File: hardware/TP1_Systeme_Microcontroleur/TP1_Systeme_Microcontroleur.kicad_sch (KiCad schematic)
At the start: 11 parts, among them U1 STM32L021K4Tx

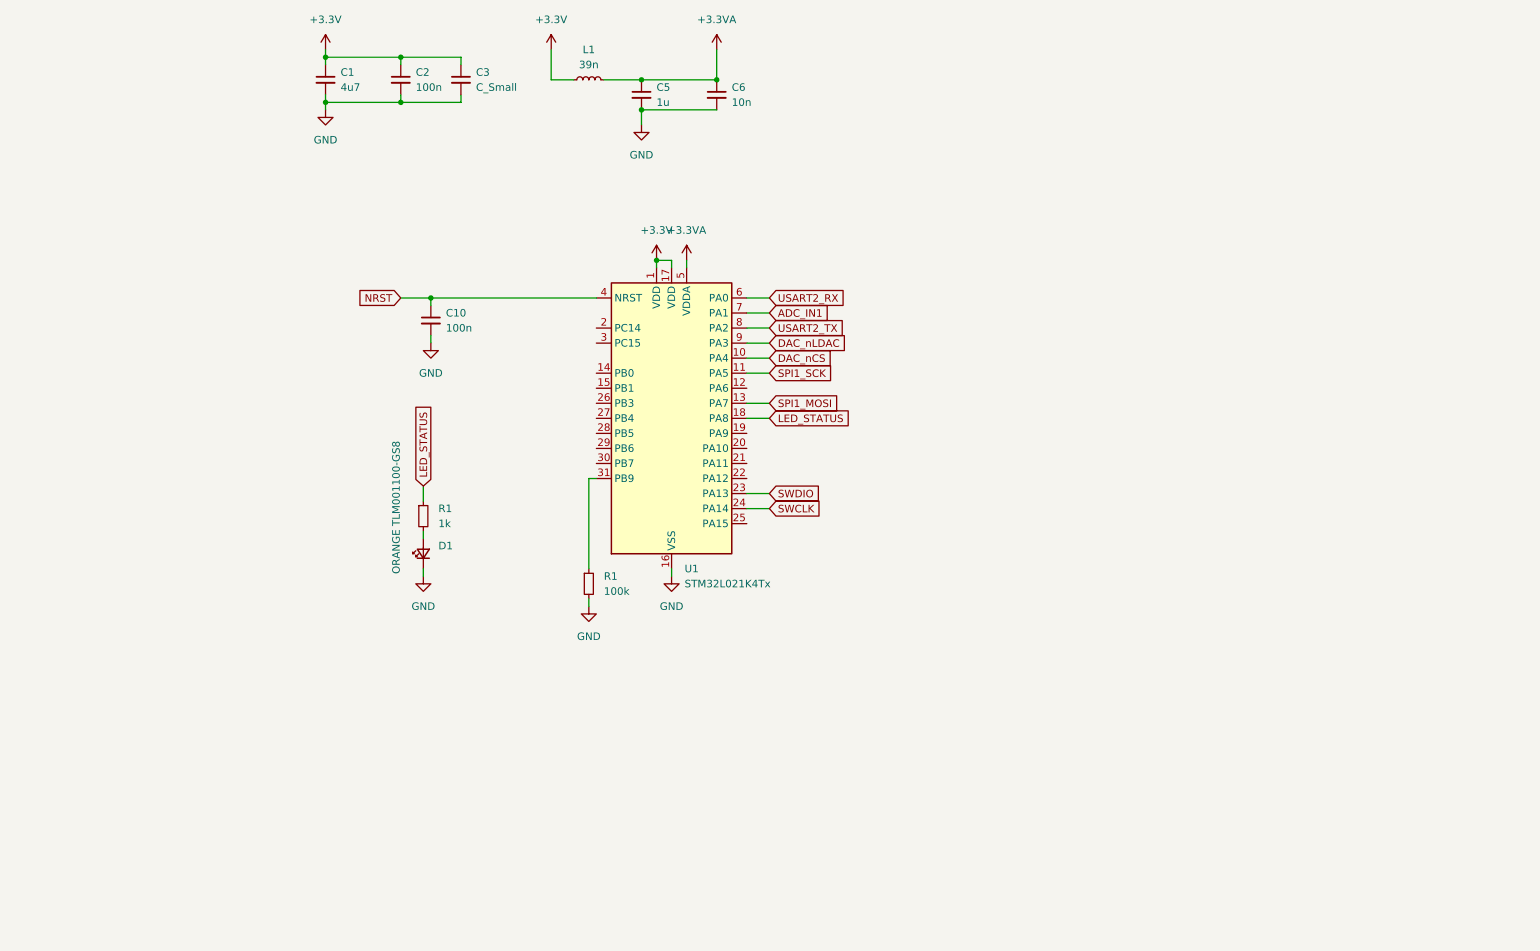
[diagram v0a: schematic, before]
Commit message: upload
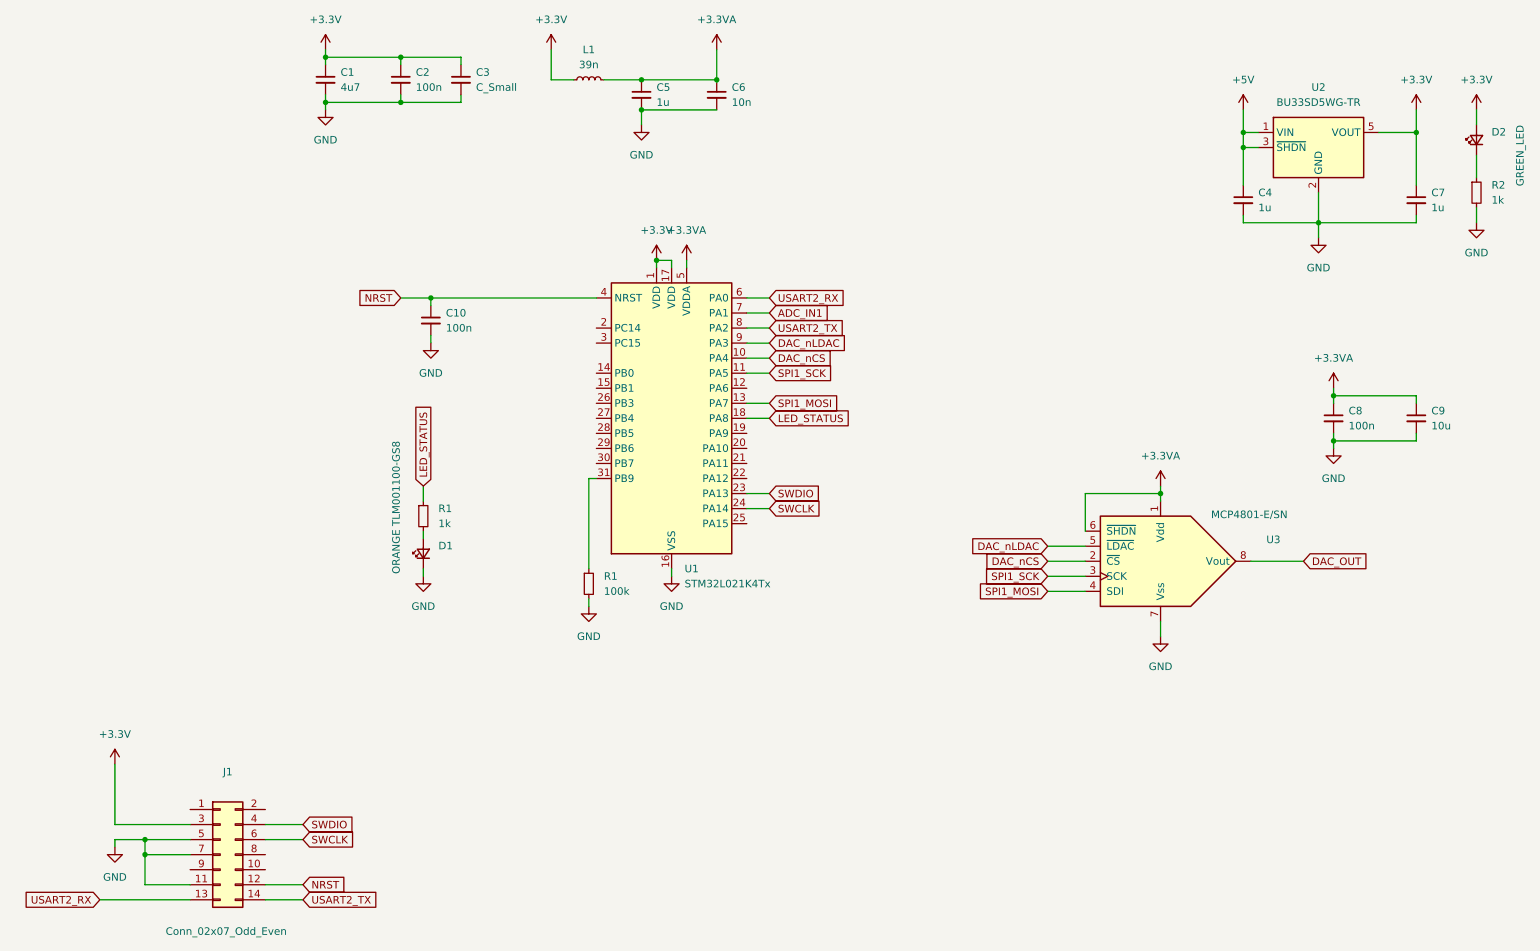
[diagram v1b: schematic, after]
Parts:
- added C4, C7: 1u, symbol Device:C_Small
- added C8: 100n, symbol Device:C_Small
- added C9: 10u, symbol Device:C_Small
- added D2: GREEN_LED, symbol Device:LED_Small
- added J1: Conn_02x07_Odd_Even, symbol Connector_Generic:Conn_02x07_Odd_Even
- added R2: 1k, symbol Device:R_Small
- added U2: BU33SD5WG-TR, Package_TO_SOT_SMD:SOT-23-5, symbol Regulator_Linear:MCP1802x-xx02xOT
- added U3: MCP4801-E/SN, symbol Analog_DAC:MCP4801
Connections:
- net +3.3V: now also C7.1, D2.2 (A), J1.3 (Pin_3), U2.5 (VOUT)
- net +3.3VA: now also C8.1, C9.1, U3.1 (Vdd), U3.6 (~{SHDN})
- net DAC_nCS: now also U3.2 (~{CS})
- net DAC_nLDAC: now also U3.5 (~{LDAC})
- net GND: now also C4.2, C7.2, C8.2, C9.2, J1.11 (Pin_11), J1.5 (Pin_5), J1.7 (Pin_7), R2.2, U2.2 (GND), U3.7 (Vss)
- net NRST: now also J1.12 (Pin_12)
- net SPI1_MOSI: now also U3.4 (SDI)
- net SPI1_SCK: now also U3.3 (SCK)
- net SWCLK: now also J1.6 (Pin_6)
- net SWDIO: now also J1.4 (Pin_4)
- net USART2_RX: now also J1.13 (Pin_13)
- net USART2_TX: now also J1.14 (Pin_14)
- new net: D2.1 (K), R2.1
- new net +5V: C4.1, U2.1 (VIN), U2.3 (~{SHDN})
- new net DAC_OUT: U3.8 (Vout)
